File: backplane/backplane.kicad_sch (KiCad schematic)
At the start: 17 parts

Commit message: FS1-3 + FS2-4
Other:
- moved on the sheet: CONECTOR_FS1_3, CONECTOR_FS2_4

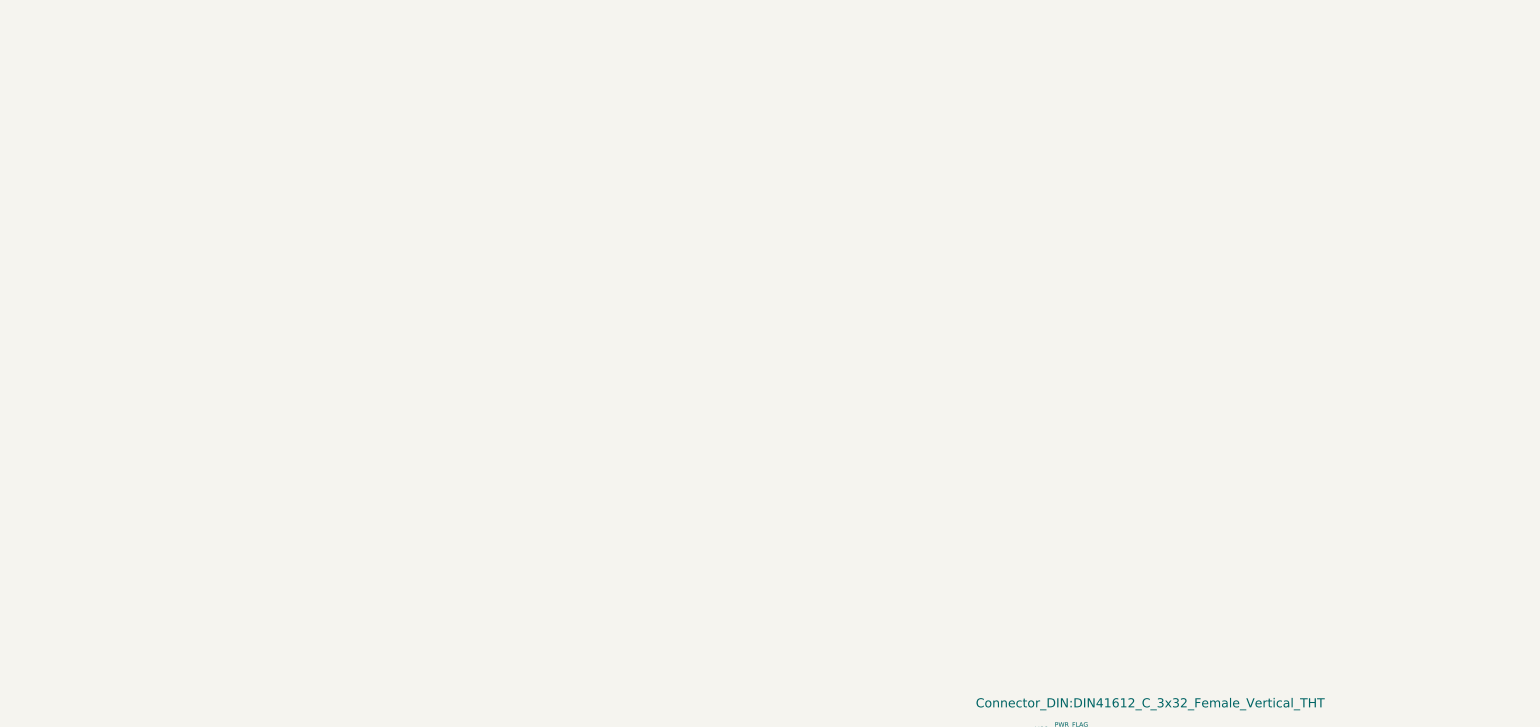
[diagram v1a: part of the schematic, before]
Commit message: backplane
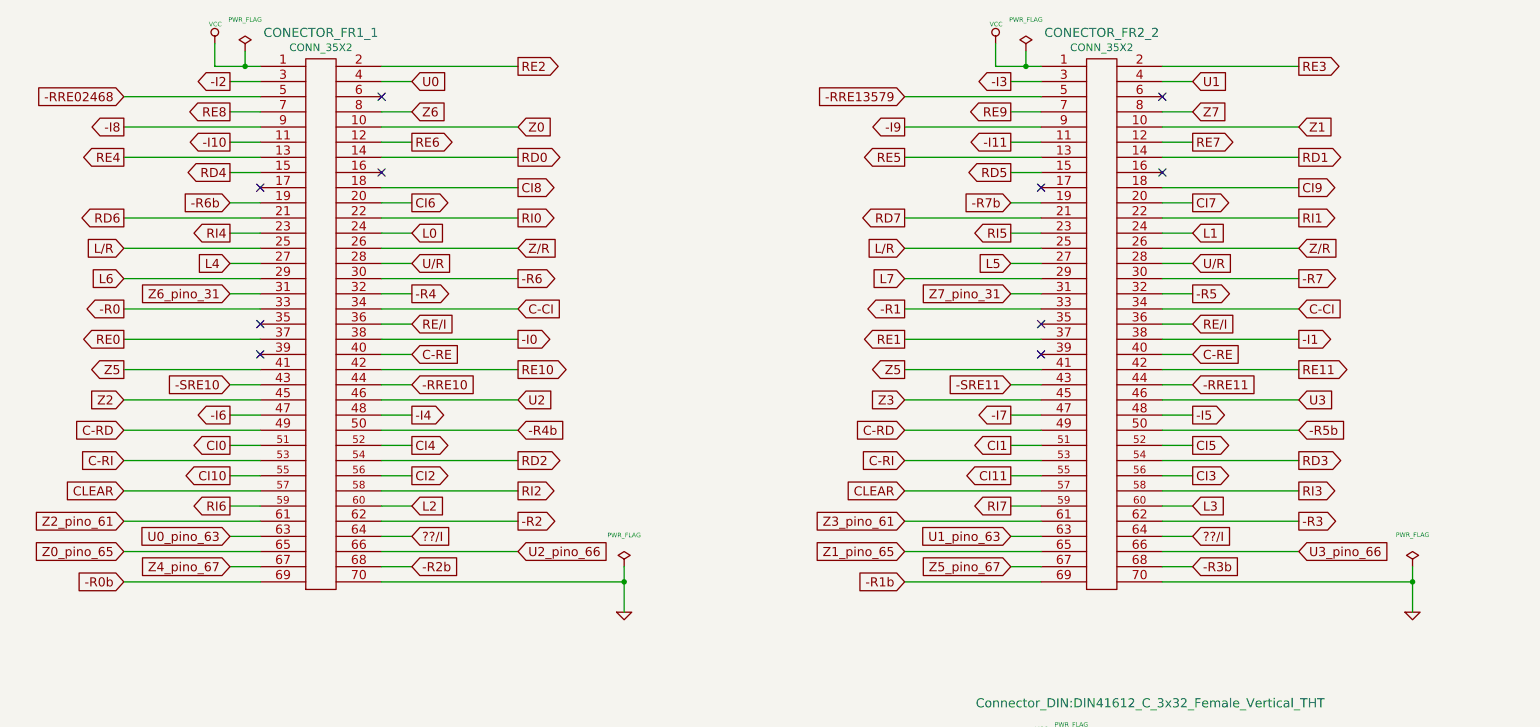
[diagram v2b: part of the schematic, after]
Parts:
- added CONECTOR_FR1_1, CONECTOR_FR2_2: CONN_35X2, symbol FR1-1-rescue:CONN_35X2-conn_35x2
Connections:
- net GND: now also CONECTOR_FR1_1.70 (P70), CONECTOR_FR2_2.70 (P70)
- net VCC: now also CONECTOR_FR1_1.1 (P1), CONECTOR_FR2_2.1 (P1)
- new net -I0: CONECTOR_FR1_1.38 (P38)
- new net -I1: CONECTOR_FR2_2.38 (P38)
- new net -I10: CONECTOR_FR1_1.11 (P11)
- new net -I11: CONECTOR_FR2_2.11 (P11)
- new net -I2: CONECTOR_FR1_1.3 (P3)
- new net -I3: CONECTOR_FR2_2.3 (P3)
- new net -I4: CONECTOR_FR1_1.48 (P48)
- new net -I5: CONECTOR_FR2_2.48 (P48)
- new net -I6: CONECTOR_FR1_1.47 (P47)
- new net -I7: CONECTOR_FR2_2.47 (P47)
- new net -I8: CONECTOR_FR1_1.9 (P9)
- new net -I9: CONECTOR_FR2_2.9 (P9)
- new net -R0: CONECTOR_FR1_1.33 (P33)
- new net -R0b: CONECTOR_FR1_1.69 (P69)
- new net -R1: CONECTOR_FR2_2.33 (P33)
- new net -R1b: CONECTOR_FR2_2.69 (P69)
- new net -R2: CONECTOR_FR1_1.62 (P62)
- new net -R2b: CONECTOR_FR1_1.68 (P68)
- new net -R3: CONECTOR_FR2_2.62 (P62)
- new net -R3b: CONECTOR_FR2_2.68 (P68)
- new net -R4: CONECTOR_FR1_1.32 (P32)
- new net -R4b: CONECTOR_FR1_1.50 (P50)
- new net -R5: CONECTOR_FR2_2.32 (P32)
- new net -R5b: CONECTOR_FR2_2.50 (P50)
- new net -R6: CONECTOR_FR1_1.30 (P30)
- new net -R6b: CONECTOR_FR1_1.19 (P19)
- new net -R7: CONECTOR_FR2_2.30 (P30)
- new net -R7b: CONECTOR_FR2_2.19 (P19)
- new net -RRE02468: CONECTOR_FR1_1.5 (P5)
- new net -RRE10: CONECTOR_FR1_1.44 (P44)
- new net -RRE11: CONECTOR_FR2_2.44 (P44)
- new net -RRE13579: CONECTOR_FR2_2.5 (P5)
- new net -SRE10: CONECTOR_FR1_1.43 (P43)
- new net -SRE11: CONECTOR_FR2_2.43 (P43)
- new net ??/I: CONECTOR_FR1_1.64 (P64), CONECTOR_FR2_2.64 (P64)
- new net C-CI: CONECTOR_FR1_1.34 (P34), CONECTOR_FR2_2.34 (P34)
- new net C-RD: CONECTOR_FR1_1.49 (P49), CONECTOR_FR2_2.49 (P49)
- new net C-RE: CONECTOR_FR1_1.40 (P40), CONECTOR_FR2_2.40 (P40)
- new net C-RI: CONECTOR_FR1_1.53 (P53), CONECTOR_FR2_2.53 (P53)
- new net CI0: CONECTOR_FR1_1.51 (P51)
- new net CI1: CONECTOR_FR2_2.51 (P51)
- new net CI10: CONECTOR_FR1_1.55 (P55)
- new net CI11: CONECTOR_FR2_2.55 (P55)
- new net CI2: CONECTOR_FR1_1.56 (P56)
- new net CI3: CONECTOR_FR2_2.56 (P56)
- new net CI4: CONECTOR_FR1_1.52 (P52)
- new net CI5: CONECTOR_FR2_2.52 (P52)
- new net CI6: CONECTOR_FR1_1.20 (P20)
- new net CI7: CONECTOR_FR2_2.20 (P20)
- new net CI8: CONECTOR_FR1_1.18 (P18)
- new net CI9: CONECTOR_FR2_2.18 (P18)
- new net CLEAR: CONECTOR_FR1_1.57 (P57), CONECTOR_FR2_2.57 (P57)
- new net L0: CONECTOR_FR1_1.24 (P24)
- new net L1: CONECTOR_FR2_2.24 (P24)
- new net L2: CONECTOR_FR1_1.60 (P60)
- new net L3: CONECTOR_FR2_2.60 (P60)
- new net L4: CONECTOR_FR1_1.27 (P27)
- new net L5: CONECTOR_FR2_2.27 (P27)
- new net L6: CONECTOR_FR1_1.29 (P29)
- new net L7: CONECTOR_FR2_2.29 (P29)
- new net L/R: CONECTOR_FR1_1.25, CONECTOR_FR2_2.25
- new net RD0: CONECTOR_FR1_1.14 (P14)
- new net RD1: CONECTOR_FR2_2.14 (P14)
- new net RD2: CONECTOR_FR1_1.54 (P54)
- new net RD3: CONECTOR_FR2_2.54 (P54)
- new net RD4: CONECTOR_FR1_1.15 (P15)
- new net RD5: CONECTOR_FR2_2.15 (P15)
- new net RD6: CONECTOR_FR1_1.21 (P21)
- new net RD7: CONECTOR_FR2_2.21 (P21)
- new net RE0: CONECTOR_FR1_1.37 (P37)
- new net RE1: CONECTOR_FR2_2.37 (P37)
- new net RE10: CONECTOR_FR1_1.42 (P42)
- new net RE11: CONECTOR_FR2_2.42 (P42)
- new net RE2: CONECTOR_FR1_1.2 (P2)
- new net RE3: CONECTOR_FR2_2.2 (P2)
- new net RE4: CONECTOR_FR1_1.13 (P13)
- new net RE5: CONECTOR_FR2_2.13 (P13)
- new net RE6: CONECTOR_FR1_1.12 (P12)
- new net RE7: CONECTOR_FR2_2.12 (P12)
- new net RE8: CONECTOR_FR1_1.7 (P7)
- new net RE9: CONECTOR_FR2_2.7 (P7)
- new net RE/I: CONECTOR_FR1_1.36 (P36), CONECTOR_FR2_2.36 (P36)
- new net RI0: CONECTOR_FR1_1.22 (P22)
- new net RI1: CONECTOR_FR2_2.22 (P22)
- new net RI2: CONECTOR_FR1_1.58 (P58)
- new net RI3: CONECTOR_FR2_2.58 (P58)
- new net RI4: CONECTOR_FR1_1.23 (P23)
- new net RI5: CONECTOR_FR2_2.23 (P23)
- new net RI6: CONECTOR_FR1_1.59 (P59)
- new net RI7: CONECTOR_FR2_2.59 (P59)
- new net U0: CONECTOR_FR1_1.4 (P4)
- new net U0_pino_63: CONECTOR_FR1_1.63 (P63)
- new net U1: CONECTOR_FR2_2.4 (P4)
- new net U1_pino_63: CONECTOR_FR2_2.63 (P63)
- new net U2: CONECTOR_FR1_1.46 (P46)
- new net U2_pino_66: CONECTOR_FR1_1.66 (P66)
- new net U3: CONECTOR_FR2_2.46 (P46)
- new net U3_pino_66: CONECTOR_FR2_2.66 (P66)
- new net U/R: CONECTOR_FR1_1.28 (P28), CONECTOR_FR2_2.28 (P28)
- new net Z0: CONECTOR_FR1_1.10 (P10)
- new net Z0_pino_65: CONECTOR_FR1_1.65 (P65)
- new net Z1: CONECTOR_FR2_2.10 (P10)
- new net Z1_pino_65: CONECTOR_FR2_2.65 (P65)
- new net Z2: CONECTOR_FR1_1.45 (P45)
- new net Z2_pino_61: CONECTOR_FR1_1.61 (P61)
- new net Z3: CONECTOR_FR2_2.45 (P45)
- new net Z3_pino_61: CONECTOR_FR2_2.61 (P61)
- new net Z4_pino_67: CONECTOR_FR1_1.67 (P67)
- new net Z5: CONECTOR_FR1_1.41 (P41), CONECTOR_FR2_2.41 (P41)
- new net Z5_pino_67: CONECTOR_FR2_2.67 (P67)
- new net Z6: CONECTOR_FR1_1.8 (P8)
- new net Z6_pino_31: CONECTOR_FR1_1.31 (P31)
- new net Z7: CONECTOR_FR2_2.8 (P8)
- new net Z7_pino_31: CONECTOR_FR2_2.31 (P31)
- new net Z/R: CONECTOR_FR1_1.26 (P26), CONECTOR_FR2_2.26 (P26)
- no-connect marks 317 -> 327
